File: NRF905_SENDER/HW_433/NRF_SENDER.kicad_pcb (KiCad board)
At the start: 2 copper layers, 76 x 51 mm, 61 parts, among them J1 SWD, J2 Conn_Coaxial, Q1 IRLML6402, SW1 SW_Push, SW2 SW_Push, U1 STM32L051C6Tx, U2 BME280, U3 NRF905, U4 MAX1724, Y1 Crystal

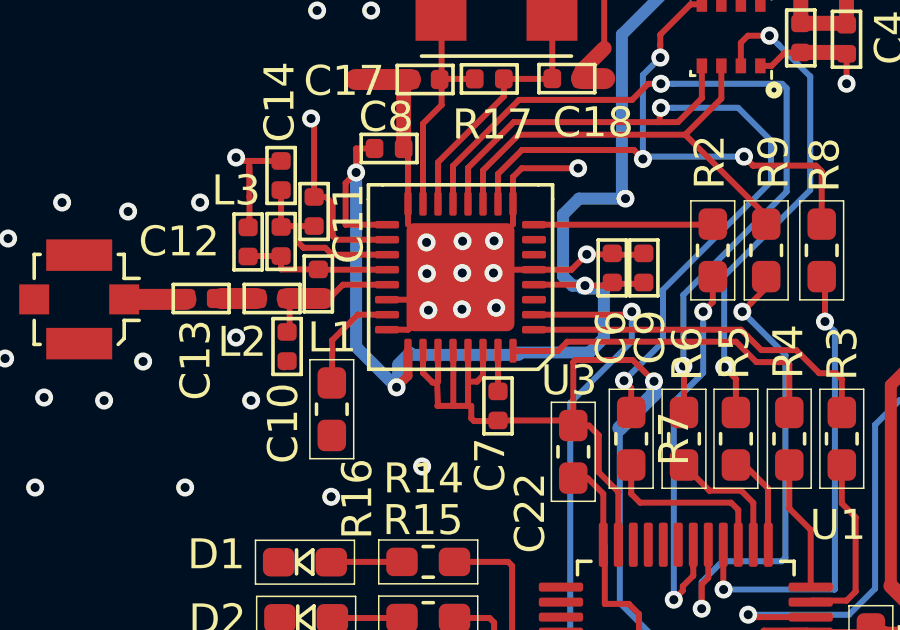
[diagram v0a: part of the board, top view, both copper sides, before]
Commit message: Change ESP32
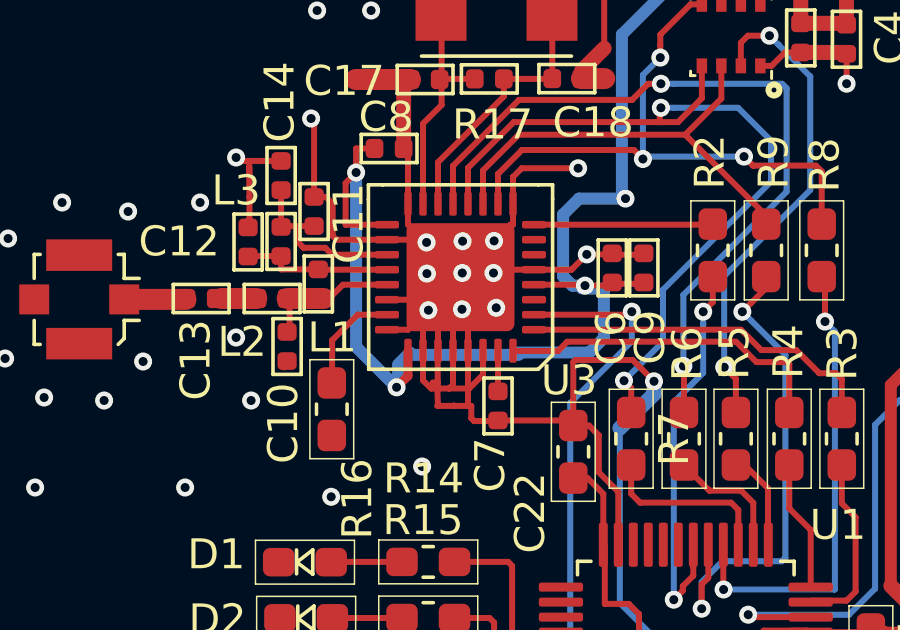
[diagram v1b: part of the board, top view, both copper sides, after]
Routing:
- net GND: track 142.7 -> 157.1 mm
